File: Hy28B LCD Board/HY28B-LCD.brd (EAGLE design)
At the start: 86.5 x 69.5 mm, 32 parts, among them K2 PIN20X2, U2 EEPROM24, X1 RASPI_BOARD_B+_F

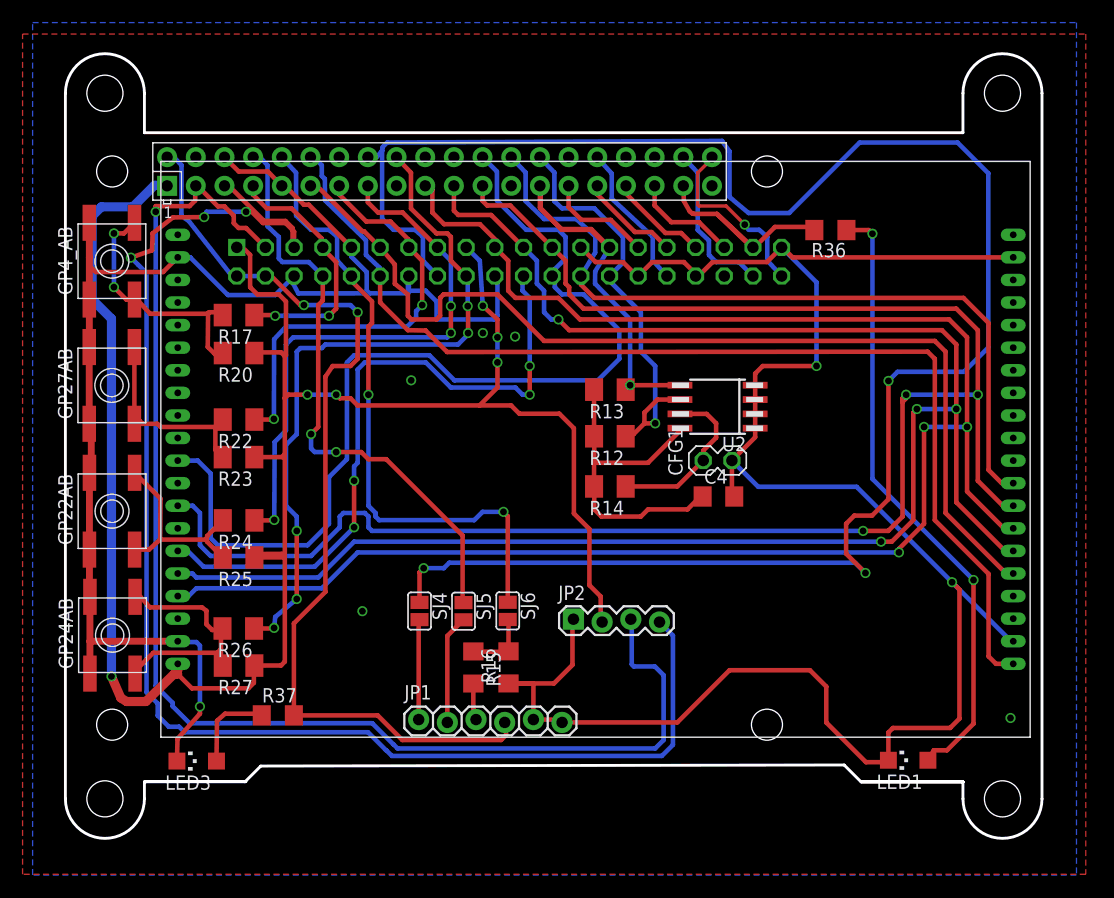
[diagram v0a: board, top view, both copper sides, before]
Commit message: HY28 and Ramps1.5
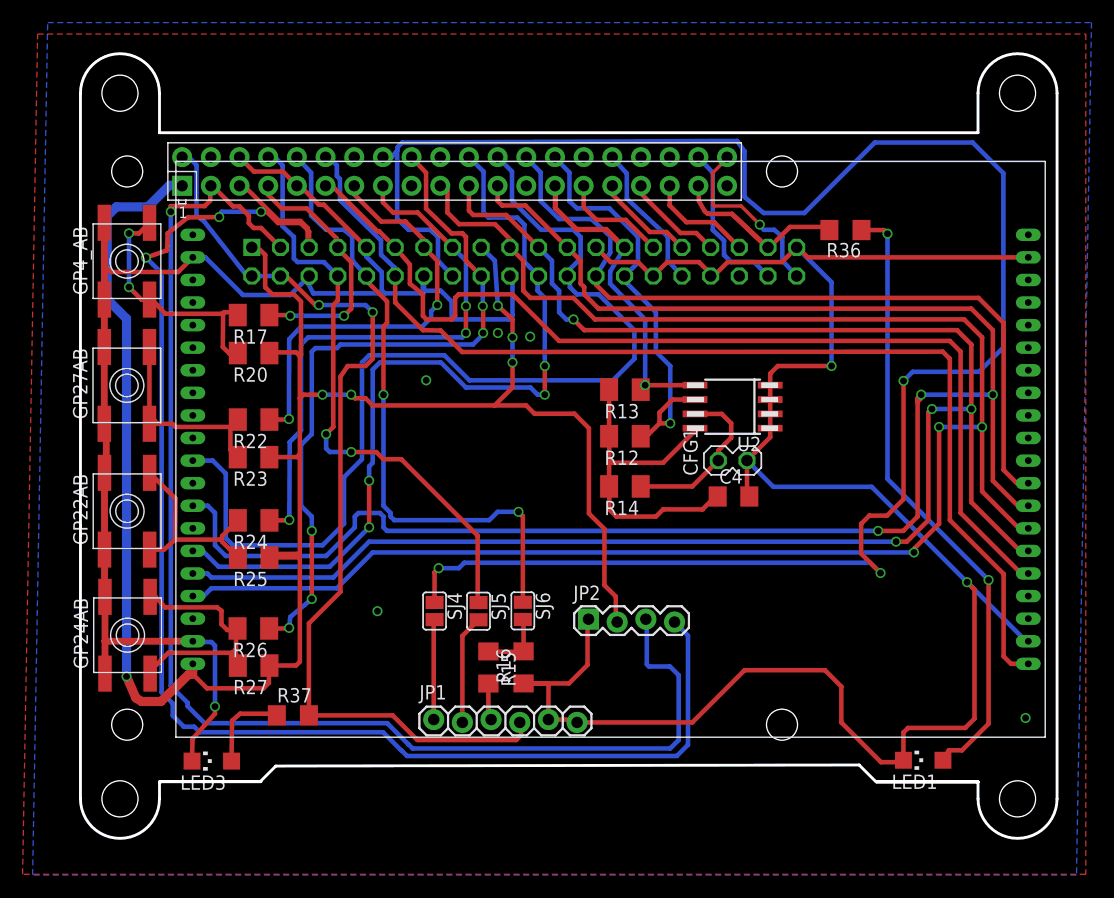
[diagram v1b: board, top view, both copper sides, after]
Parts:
- moved C4 1.33 mm to (60.4, 31.1)
- moved CFG1 1.33 mm to (59.0, 34.3)
- moved JP1 1.33 mm to (33.8, 11.4)
- moved JP2 1.33 mm to (47.5, 20.1)
- moved K2 1.33 mm to (41.8, 51.9)
- moved LED1 1.33 mm to (77.2, 7.75)
- moved R15 1.33 mm to (38.7, 16.0)
- moved R16 1.33 mm to (41.8, 16.0)
- moved R17 1.33 mm to (17.9, 47.2)
- moved R22 1.33 mm to (17.9, 37.9)
- moved R23 1.33 mm to (17.9, 34.6)
- moved R24 1.33 mm to (17.9, 29.0)
- moved R25 1.33 mm to (17.9, 25.7)
- moved R27 1.33 mm to (17.9, 16.1)
- moved R36 1.33 mm to (70.3, 54.7)
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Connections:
- net GPIO25: now also K2.22
- net GPIO28: no longer K2.22
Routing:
- net GPIO25: track 0.00 -> 14.6 mm
